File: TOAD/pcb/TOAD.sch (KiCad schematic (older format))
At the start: 151 parts, among them IC1 STM32F405RxTx, IC10 ADP3335, IC11 CS2100-CP, IC12 BGS12AL7, IC13 SL18860DC, IC2 Si4463, IC3 MAX-M8Q, IC4 SN74LVC1G0832, IC5 BGS12AL7, IC6 ADP3335, IC7 BQ24232HA, IC8 NC7SZ04, IC9 Si4463, J1 USB, J2 BATT, J3 SWITCH, P1 SMA, P2 SWD_TC, P3 SMA, P4 SMA, U1 MICROSD, X1 USB Cap, X10 RF Frame, X11 RF Cover, X12 Mount, X13 Mount, X14 RF Frame, X15 RF Cover, X2 USB Mini-B, X3 Case, X4 SMA Panel, X5 SMA Panel, X6 PWR Switch, X7 Battery, X8 Mount, X9 Mount, Y1 26M TCXO

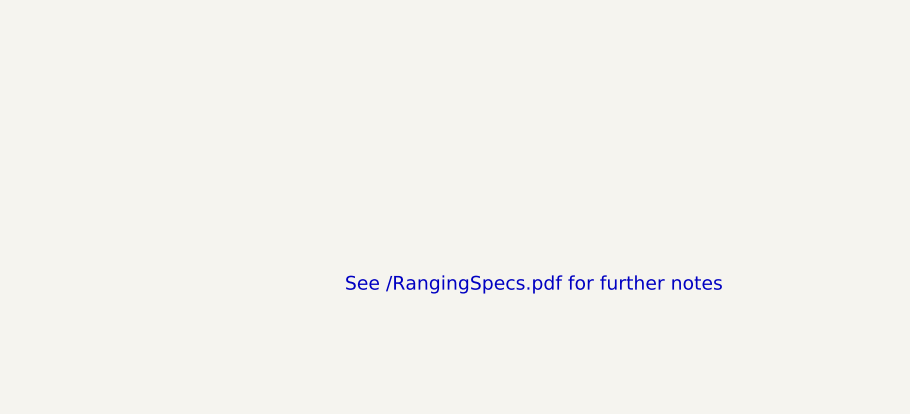
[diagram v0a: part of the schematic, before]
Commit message: folder organisation and BOM
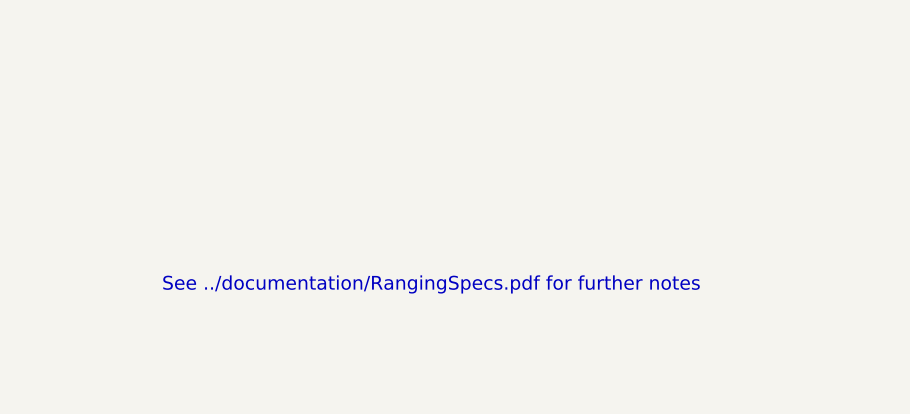
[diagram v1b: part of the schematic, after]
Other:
- note added: "See ../documentation/RangingSpecs.pdf for further notes"
- note removed: "See /RangingSpecs.pdf for further notes"
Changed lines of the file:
@@
 	0    -1   -1   0
 $EndComp
-Text Notes 14100 10750 0    60   ~ 0
-See /RangingSpecs.pdf for further notes
+Text Notes 13300 10750 0    60   ~ 0
+See ../documentation/RangingSpecs.pdf for further notes
 $Comp
 L C_Small C26
